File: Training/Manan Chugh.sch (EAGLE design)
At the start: 10 parts, among them IC1 NE555, J1 1X2-3.5MM

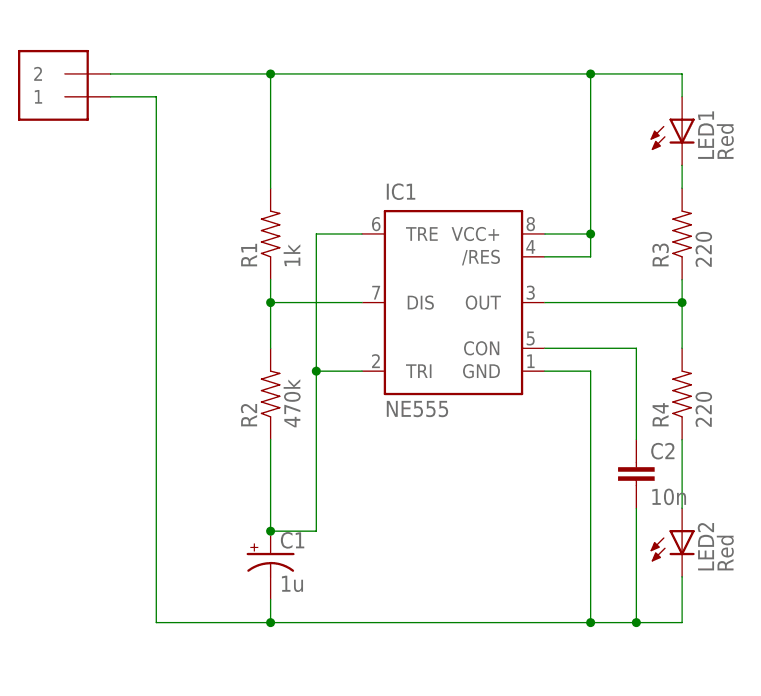
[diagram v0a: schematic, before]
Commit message: Some clean up of git
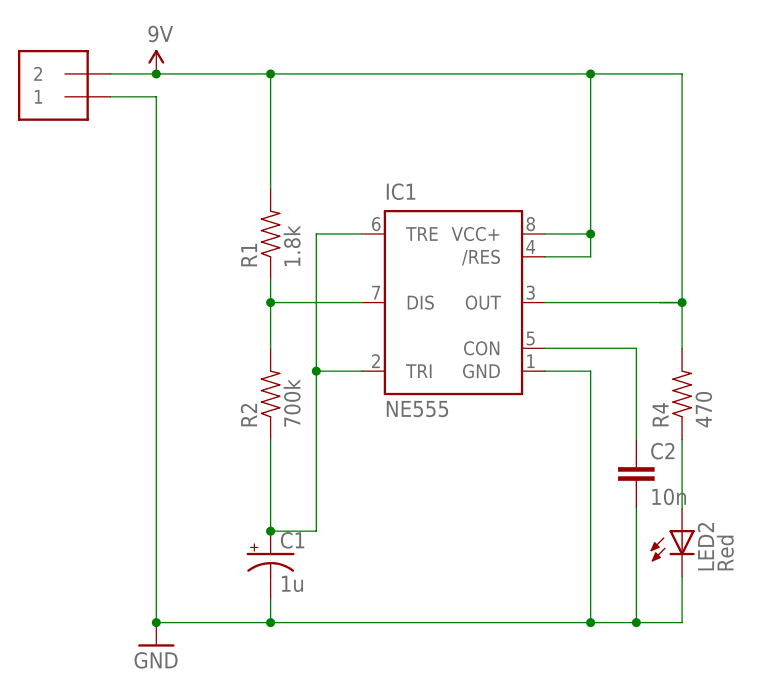
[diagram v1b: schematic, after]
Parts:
- removed LED1: Red, adafruit:LED5MM
- removed R3: 220, SparkFun-Resistors:RESISTORAXIAL-0.3
- R1: value 1k -> 1.8k
- R2: value 470k -> 700k
- R4: value 220 -> 470
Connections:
- removed net N$3: LED1.C, R3.2
- removed net N$4: IC1.OUT, R3.1, R4.2
- net VCC+: now also IC1.OUT, R4.2; no longer LED1.A
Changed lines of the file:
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@@
 <parts>
 <part name="IC1" library="st-microelectronics" deviceset="NE555" device=""/>
-<part name="R1" library="SparkFun-Resistors" deviceset="RESISTOR" device="AXIAL-0.3" value="1k"/>
-<part name="R2" library="SparkFun-Resistors" deviceset="RESISTOR" device="AXIAL-0.3" value="470k"/>
-<part name="R3" library="SparkFun-Resistors" deviceset="RESISTOR" device="AXIAL-0.3" value="220"/>
-<part name="R4" library="SparkFun-Resistors" deviceset="RESISTOR" device="AXIAL-0.3" value="220"/>
+<part name="R1" library="SparkFun-Resistors" deviceset="RESISTOR" device="AXIAL-0.3" value="1.8k"/>
+<part name="R2" library="SparkFun-Resistors" deviceset="RESISTOR" device="AXIAL-0.3" value="700k"/>
+<part name="R4" library="SparkFun-Resistors" deviceset="RESISTOR" device="AXIAL-0.3" value="470"/>
 <part name="C1" library="SparkFun-Capacitors" deviceset="CAP_POL" device="PTH2" value="1u"/>
-<part name="LED1" library="adafruit" deviceset="LED" device="5MM" value="Red"/>
 <part name="LED2" library="adafruit" deviceset="LED" device="5MM" value="Red"/>
 <part name="J1" library="adafruit" deviceset="1X2" device="-3.5MM"/>
 <part name="C2" library="SparkFun-Capacitors" deviceset="CAP" device="PTH" value="10n"/>
+<part name="GND" library="SparkFun-Aesthetics" deviceset="GND" device=""/>
+<part name="VCC+" library="SparkFun-Aesthetics" deviceset="VCC" device="" value="9V"/>
 </parts>
 <sheets>
@@
 <instance part="R1" gate="G$1" x="-33.02" y="73.66" rot="R90"/>
 <instance part="R2" gate="G$1" x="-33.02" y="55.88" rot="R90"/>
-<instance part="R3" gate="G$1" x="12.7" y="73.66" rot="R90"/>
 <instance part="R4" gate="G$1" x="12.7" y="55.88" rot="R90"/>
 <instance part="C1" gate="G$1" x="-33.02" y="38.1"/>
-<instance part="LED1" gate="G$1" x="12.7" y="86.36"/>
 <instance part="LED2" gate="G$1" x="12.7" y="40.64"/>
 <instance part="J1" gate="G$1" x="-55.88" y="91.44" rot="R180"/>
 <instance part="C2" gate="G$1" x="7.62" y="45.72"/>
+<instance part="GND" gate="1" x="-45.72" y="27.94"/>
+<instance part="VCC+" gate="G$1" x="-45.72" y="91.44"/>
 </instances>
 <busses>
 </busses>
 <nets>
-<net name="VCC+" class="0">
-<segment>
-<pinref part="J1" gate="G$1" pin="2"/>
-<wire x1="-50.8" y1="91.44" x2="-33.02" y2="91.44" width="0.1524" layer="91"/>
-<wire x1="-33.02" y1="91.44" x2="2.54" y2="91.44" width="0.1524" layer="91"/>
-<pinref part="R1" gate="G$1" pin="2"/>
-<wire x1="-33.02" y1="78.74" x2="-33.02" y2="91.44" width="0.1524" layer="91"/>
-<junction x="-33.02" y="91.44"/>
-<pinref part="IC1" gate="G$1" pin="/RES"/>
-<wire x1="-2.54" y1="71.12" x2="2.54" y2="71.12" width="0.1524" layer="91"/>
-<wire x1="2.54" y1="71.12" x2="2.54" y2="73.66" width="0.1524" layer="91"/>
-<pinref part="IC1" gate="G$1" pin="VCC+"/>
-<wire x1="2.54" y1="73.66" x2="2.54" y2="91.44" width="0.1524" layer="91"/>
-<wire x1="-2.54" y1="73.66" x2="2.54" y2="73.66" width="0.1524" layer="91"/>
-<junction x="2.54" y="73.66"/>
-<wire x1="2.54" y1="91.44" x2="12.7" y2="91.44" width="0.1524" layer="91"/>
-<junction x="2.54" y="91.44"/>
-<pinref part="LED1" gate="G$1" pin="A"/>
-<wire x1="12.7" y1="91.44" x2="12.7" y2="88.9" width="0.1524" layer="91"/>
-</segment>
-</net>
-<net name="N$4" class="0">
-<segment>
-<pinref part="R3" gate="G$1" pin="1"/>
-<pinref part="R4" gate="G$1" pin="2"/>
-<wire x1="12.7" y1="68.58" x2="12.7" y2="66.04" width="0.1524" layer="91"/>
-<pinref part="IC1" gate="G$1" pin="OUT"/>
-<wire x1="12.7" y1="66.04" x2="12.7" y2="60.96" width="0.1524" layer="91"/>
-<wire x1="-2.54" y1="66.04" x2="12.7" y2="66.04" width="0.1524" layer="91"/>
-<junction x="12.7" y="66.04"/>
-</segment>
-</net>
 <net name="N$7" class="0">
 <segment>
@@
 <wire x1="-22.86" y1="66.04" x2="-33.02" y2="66.04" width="0.1524" layer="91"/>
 <junction x="-33.02" y="66.04"/>
-</segment>
-</net>
-<net name="N$3" class="0">
-<segment>
-<pinref part="LED1" gate="G$1" pin="C"/>
-<pinref part="R3" gate="G$1" pin="2"/>
-<wire x1="12.7" y1="81.28" x2="12.7" y2="78.74" width="0.1524" layer="91"/>
 </segment>
 </net>
@@
 <wire x1="7.62" y1="43.18" x2="7.62" y2="30.48" width="0.1524" layer="91"/>
 <junction x="7.62" y="30.48"/>
+<pinref part="GND" gate="1" pin="GND"/>
+<junction x="-45.72" y="30.48"/>
 </segment>
 </net>
@@
 </segment>
 </net>
+<net name="VCC+" class="0">
+<segment>
+<pinref part="J1" gate="G$1" pin="2"/>
+<wire x1="-50.8" y1="91.44" x2="-45.72" y2="91.44" width="0.1524" layer="91"/>
+<wire x1="-45.72" y1="91.44" x2="-33.02" y2="91.44" width="0.1524" layer="91"/>
+<wire x1="-33.02" y1="91.44" x2="2.54" y2="91.44" width="0.1524" layer="91"/>
+<pinref part="R1" gate="G$1" pin="2"/>
+<wire x1="-33.02" y1="78.74" x2="-33.02" y2="91.44" width="0.1524" layer="91"/>
+<junction x="-33.02" y="91.44"/>
+<pinref part="IC1" gate="G$1" pin="/RES"/>
+<wire x1="-2.54" y1="71.12" x2="2.54" y2="71.12" width="0.1524" layer="91"/>
+<wire x1="2.54" y1="71.12" x2="2.54" y2="73.66" width="0.1524" layer="91"/>
+<pinref part="IC1" gate="G$1" pin="VCC+"/>
+<wire x1="2.54" y1="73.66" x2="2.54" y2="91.44" width="0.1524" layer="91"/>
+<wire x1="-2.54" y1="73.66" x2="2.54" y2="73.66" width="0.1524" layer="91"/>
+<junction x="2.54" y="73.66"/>
+<wire x1="2.54" y1="91.44" x2="12.7" y2="91.44" width="0.1524" layer="91"/>
+<junction x="2.54" y="91.44"/>
+<pinref part="R4" gate="G$1" pin="2"/>
+<pinref part="IC1" gate="G$1" pin="OUT"/>
+<wire x1="12.7" y1="66.04" x2="12.7" y2="60.96" width="0.1524" layer="91"/>
+<wire x1="-2.54" y1="66.04" x2="12.7" y2="66.04" width="0.1524" layer="91"/>
+<wire x1="12.7" y1="91.44" x2="12.7" y2="66.04" width="0.1524" layer="91"/>
+<junction x="12.7" y="66.04"/>
+<wire x1="12.7" y1="66.04" x2="10.16" y2="66.04" width="0.1524" layer="91"/>
+<pinref part="VCC+" gate="G$1" pin="VCC"/>
+<junction x="-45.72" y="91.44"/>
+</segment>
+</net>
